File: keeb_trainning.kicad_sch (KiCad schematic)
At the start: 19 parts, among them U2 Arduino_Pro_Micro

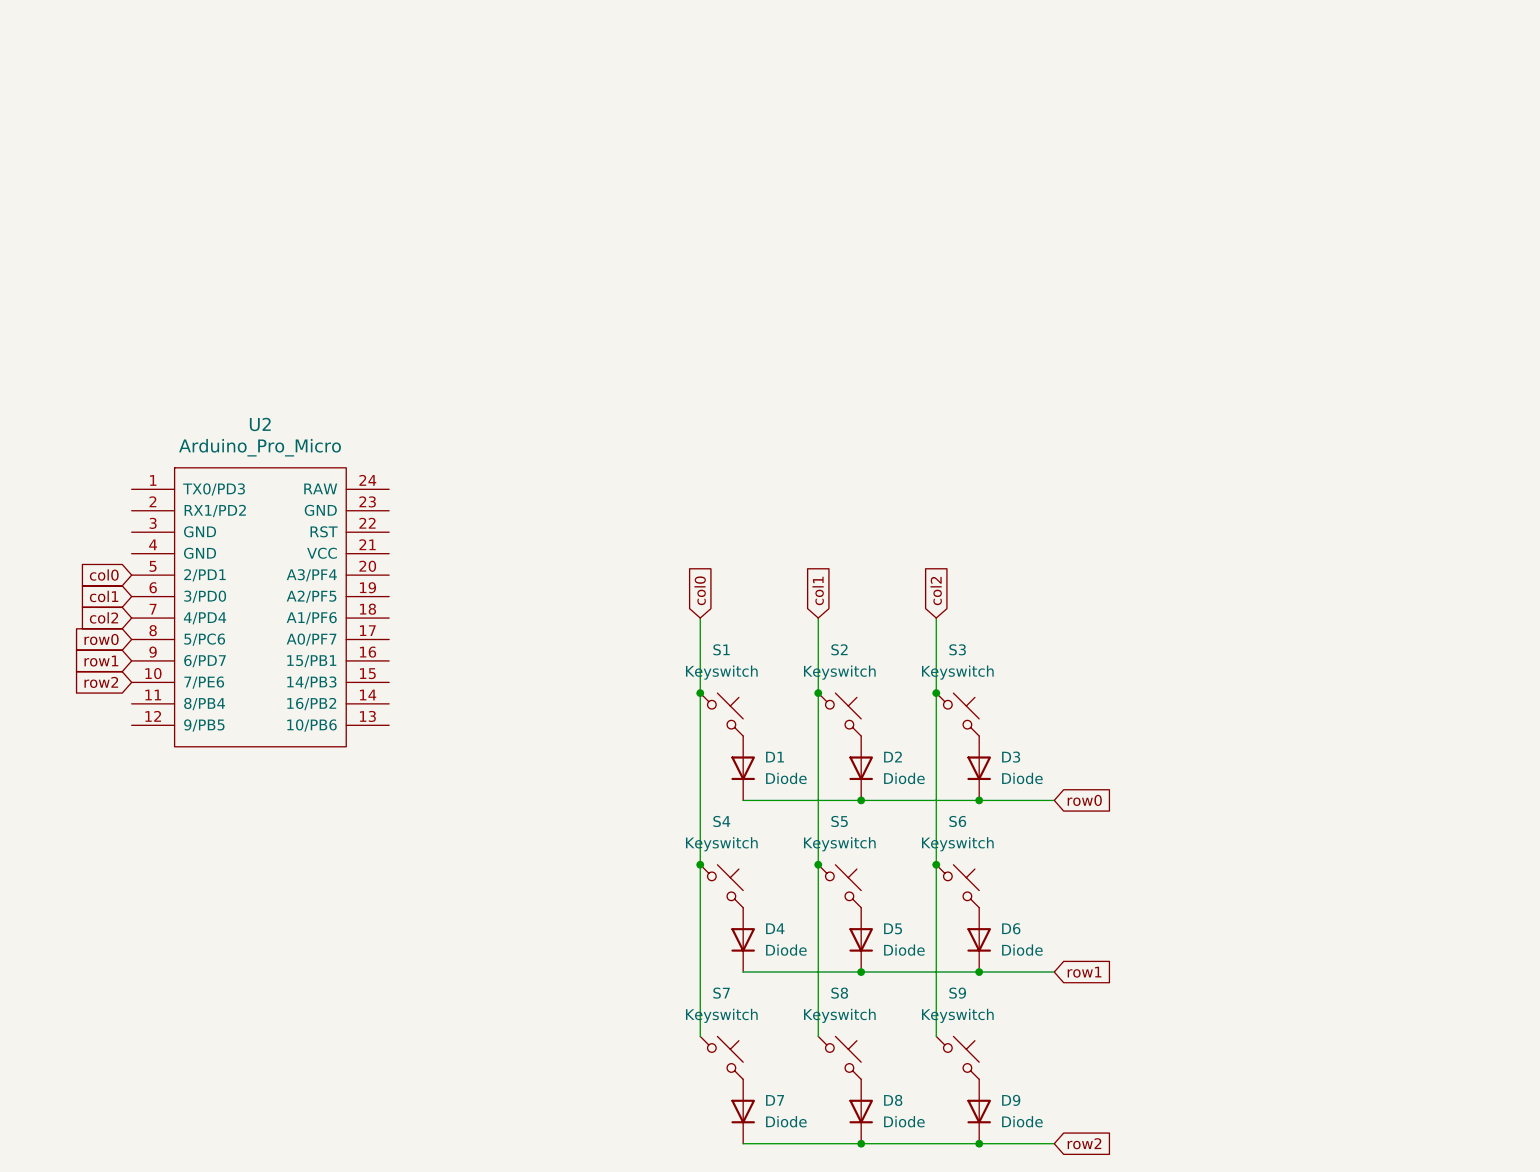
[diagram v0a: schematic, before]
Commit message: :construction: WIP: Drawing schematics
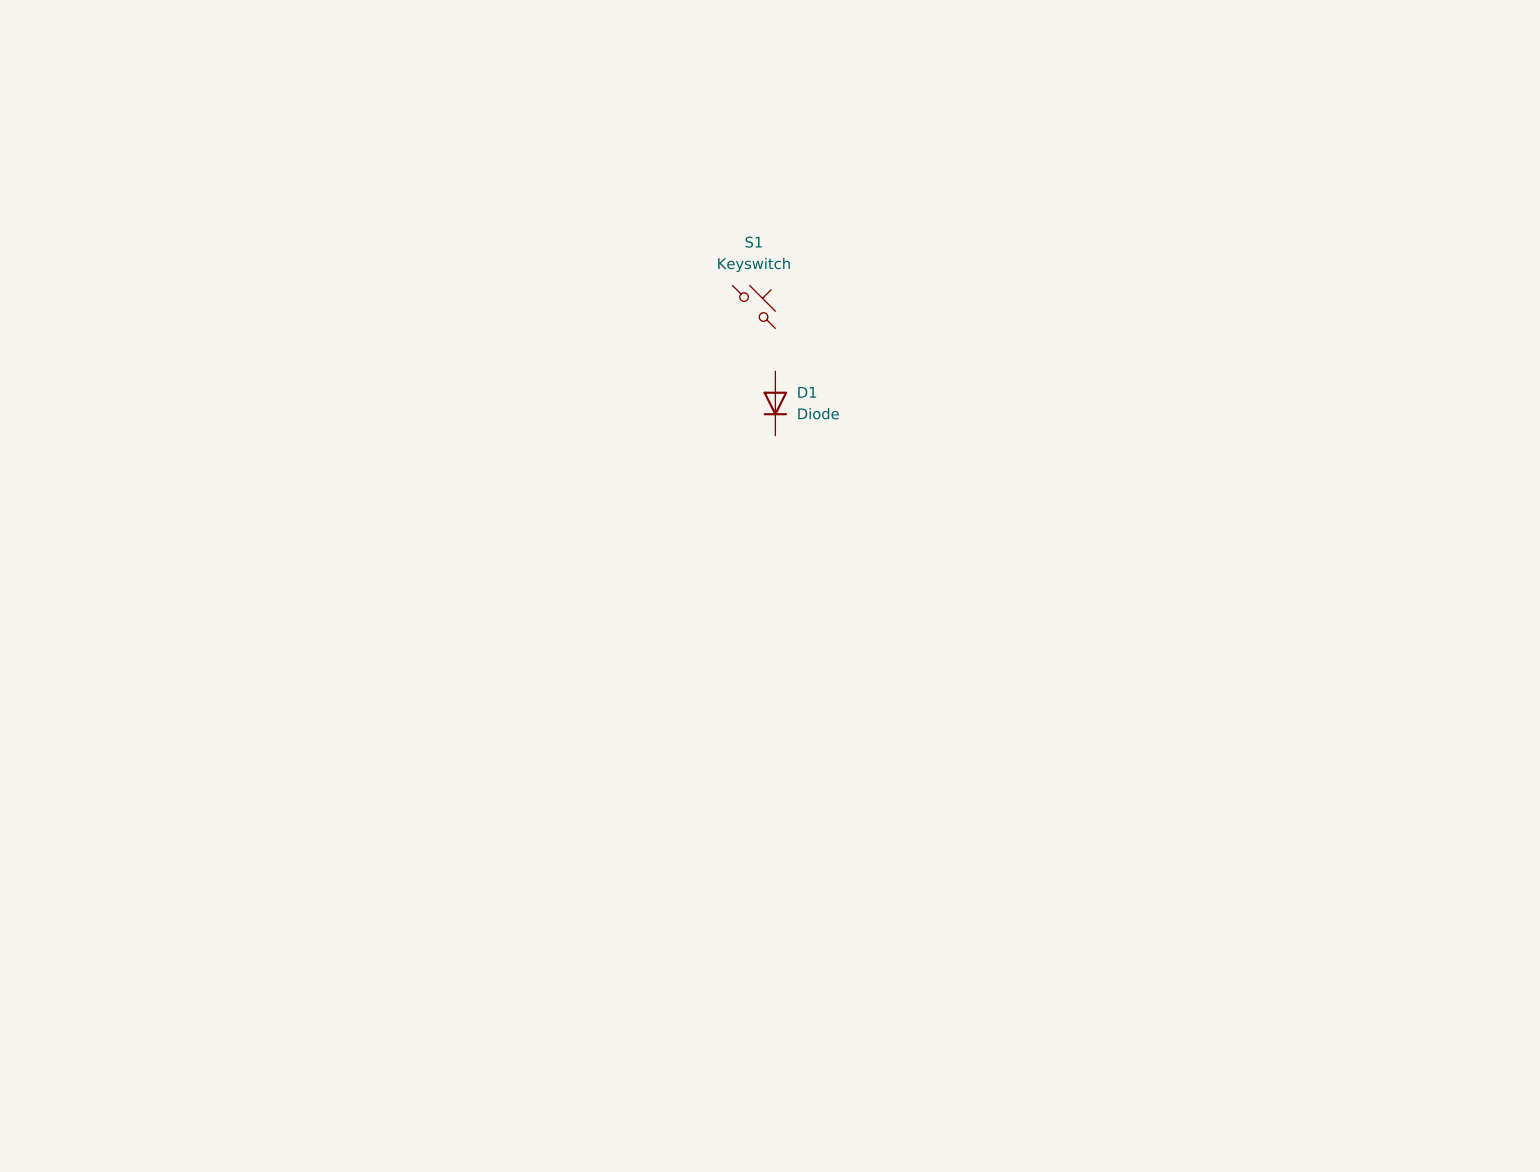
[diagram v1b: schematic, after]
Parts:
- removed D2, D3, D4, D5, D6, D7, D8, D9: Diode, ScottoKeebs_Components:Diode_DO-35, symbol ScottoKeebs:Placeholder_Diode
- removed S2, S3, S4, S5, S6, S7, S8, S9: Keyswitch, Button_Switch_Keyboard:SW_Cherry_MX_1.00u_PCB, symbol ScottoKeebs:Placeholder_Keyswitch
- removed U2: Arduino_Pro_Micro, ScottoKeebs_MCU:Arduino_Pro_Micro, symbol ScottoKeebs:MCU_Arduino_Pro_Micro
- D1: footprint ScottoKeebs_Components:Diode_DO-35 -> (none)
- S1: footprint Button_Switch_Keyboard:SW_Cherry_MX_1.00u_PCB -> (none)
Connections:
- net at D1.2 (A): no longer S1.2
- net col0: no longer names the net of S1.1
- net row0: no longer names the net of D1.1 (K)

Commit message: :construction: WIP: Redraw wires
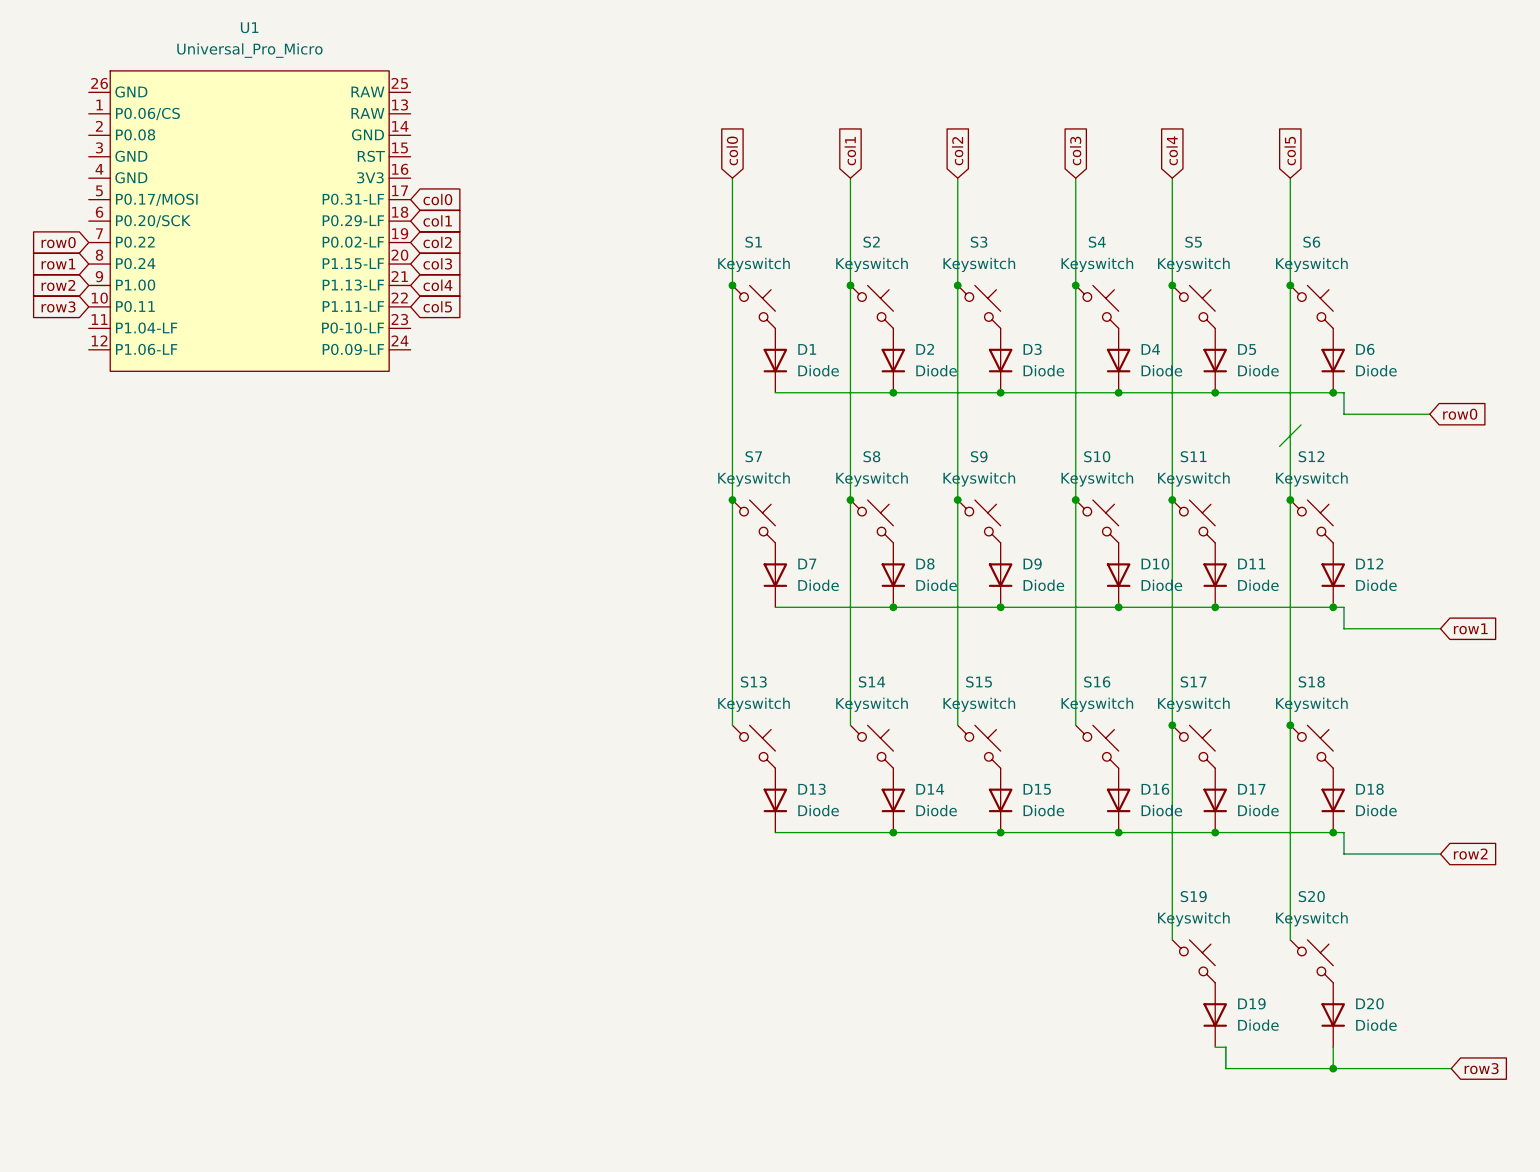
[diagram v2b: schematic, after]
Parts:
- added D10, D11, D12, D13, D14, D15, D16, D17, D18, D19, D2, D20, D3, D4, D5, D6, D7, D8, D9: Diode, ScottoKeebs_Components:Diode_SOD-123, symbol ScottoKeebs:Placeholder_Diode
- added S10, S11, S12, S13, S14, S15, S16, S17, S18, S2, S3, S4, S5, S6, S7, S8, S9: Keyswitch, ScottoKeebs_Choc:Choc_V2, symbol ScottoKeebs:Placeholder_Keyswitch
- added S19, S20: Keyswitch, ScottoKeebs_Choc:Choc_V2_1.50u_90deg, symbol ScottoKeebs:Placeholder_Keyswitch
- added U1: Universal_Pro_Micro, custom:Universal_Pro_Micro_Footprint, symbol custom:Universal_Pro_Micro_Footprint
- D1: footprint (none) -> ScottoKeebs_Components:Diode_SOD-123
- S1: footprint (none) -> ScottoKeebs_Choc:Choc_V2
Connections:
- net row0: now reaches D1.1 (K)
- net row0: now also D2.1 (K), D3.1 (K), D4.1 (K), D5.1 (K), D6.1 (K), U1.7 (P0.22)
- net at D1.2 (A): now also S1.2
- net col0: now reaches S1.1
- net col0: now also S13.1, S7.1, U1.17 (P0.31-LF)
- new net: D8.2 (A), S8.2
- new net: D17.2 (A), S17.2
- new net: D20.2 (A), S20.2
- new net: D4.2 (A), S4.2
- new net: D6.2 (A), S6.2
- new net: D13.2 (A), S13.2
- new net: D19.2 (A), S19.2
- new net: D12.2 (A), S12.2
- new net: D10.2 (A), S10.2
- new net: D3.2 (A), S3.2
- new net: D9.2 (A), S9.2
- new net: D2.2 (A), S2.2
- new net: D15.2 (A), S15.2
- new net: D14.2 (A), S14.2
- new net: D18.2 (A), S18.2
- new net: D7.2 (A), S7.2
- new net: D11.2 (A), S11.2
- new net: D5.2 (A), S5.2
- new net: D16.2 (A), S16.2
- new net col1: S14.1, S2.1, S8.1, U1.18 (P0.29-LF)
- new net col2: S15.1, S3.1, S9.1, U1.19 (P0.02-LF)
- new net col3: S10.1, S16.1, S4.1, U1.20 (P1.15-LF)
- new net col4: S11.1, S17.1, S19.1, S5.1, U1.21 (P1.13-LF)
- new net col5: S12.1, S18.1, S20.1, S6.1, U1.22 (P1.11-LF)
- new net row1: D10.1 (K), D11.1 (K), D12.1 (K), D7.1 (K), D8.1 (K), D9.1 (K), U1.8 (P0.24)
- new net row2: D13.1 (K), D14.1 (K), D15.1 (K), D16.1 (K), D17.1 (K), D18.1 (K), U1.9 (P1.00)
- new net row3: D19.1 (K), D20.1 (K), U1.10 (P0.11)
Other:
- moved on the sheet: D1

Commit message: :construction: WIP: Added hotswap
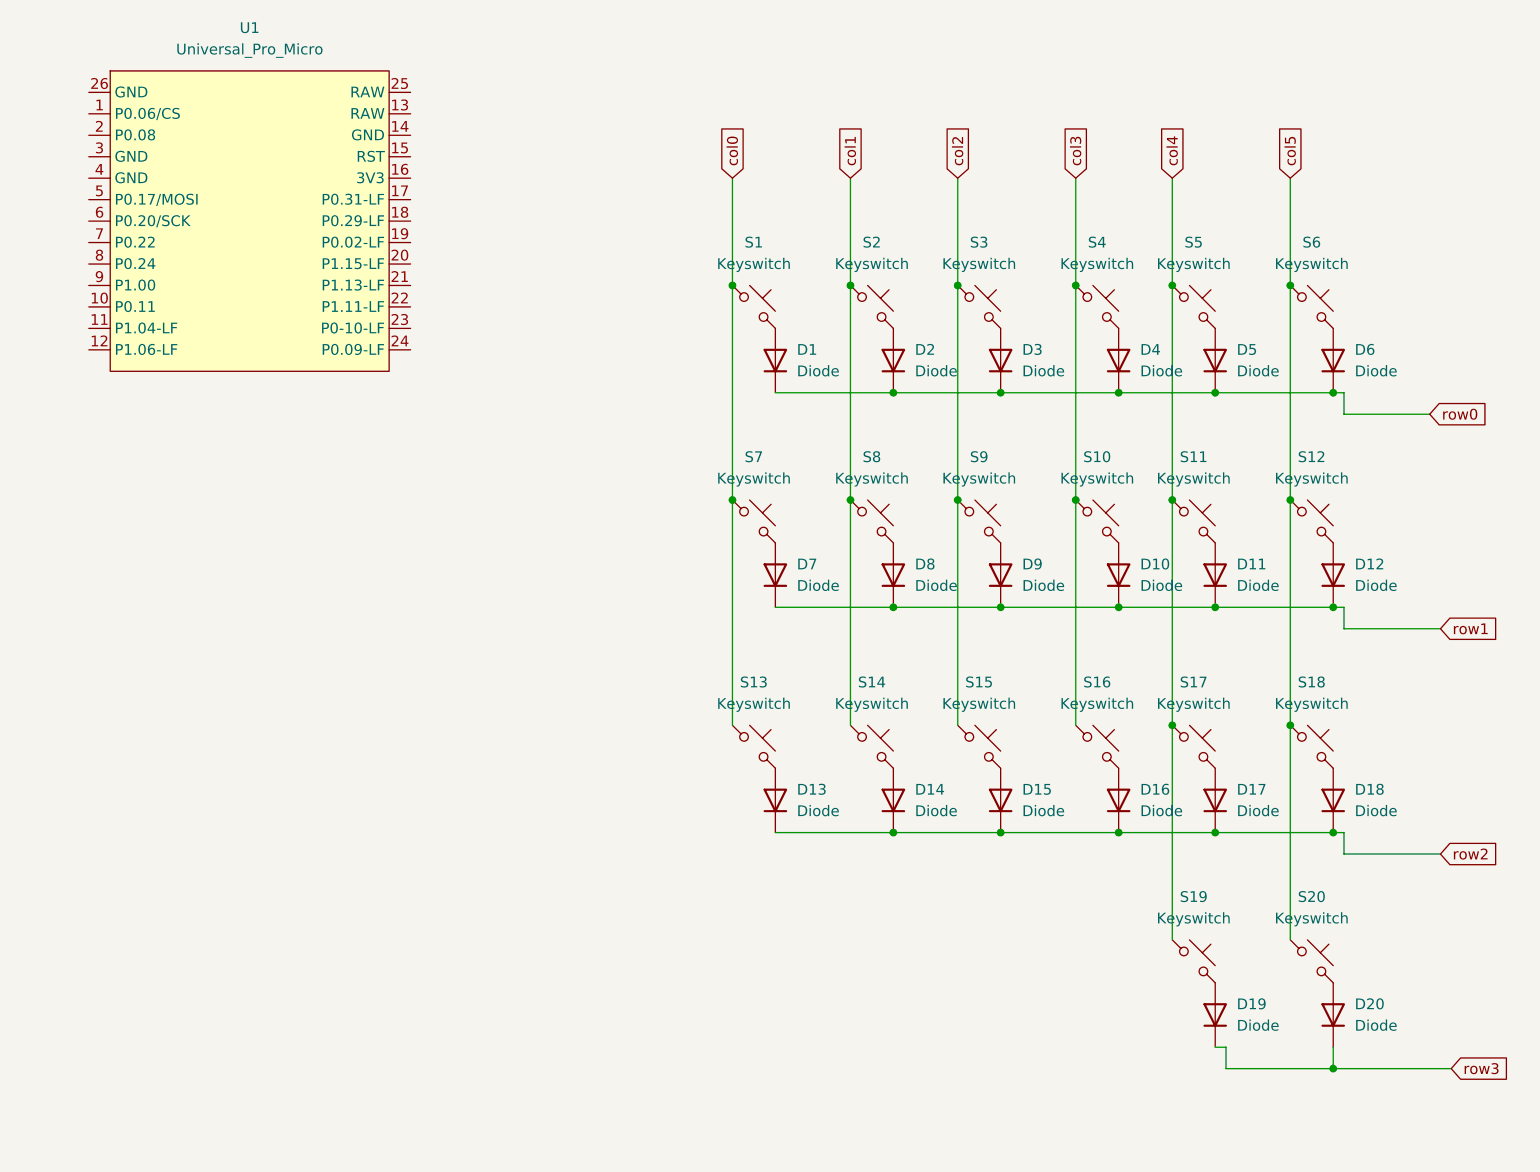
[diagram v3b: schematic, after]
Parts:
- S1, S10, S11, S12, S13, S14, S15, S16, S17, S18, S2, S3, S4, S5, S6, S7, S8, S9: footprint ScottoKeebs_Choc:Choc_V2 -> ScottoKeebs_Hotswap:Hotswap_Choc_V1
- S19, S20: footprint ScottoKeebs_Choc:Choc_V2_1.50u_90deg -> ScottoKeebs_Hotswap:Hotswap_Choc_V1
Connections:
- net col0: no longer U1.17 (P0.31-LF)
- net col1: no longer U1.18 (P0.29-LF)
- net col2: no longer U1.19 (P0.02-LF)
- net col3: no longer U1.20 (P1.15-LF)
- net col4: no longer U1.21 (P1.13-LF)
- net col5: no longer U1.22 (P1.11-LF)
- net row0: no longer U1.7 (P0.22)
- net row1: no longer U1.8 (P0.24)
- net row2: no longer U1.9 (P1.00)
- net row3: no longer U1.10 (P0.11)
